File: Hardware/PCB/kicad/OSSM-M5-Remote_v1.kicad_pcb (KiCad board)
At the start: 2 copper layers, 108.5 x 73.1 mm, 13 parts, among them M5-CORE2 M5_CORE2, U1 PCA9685PW, U2 MCP23017_SS, U3 JST-PH-2MM,180

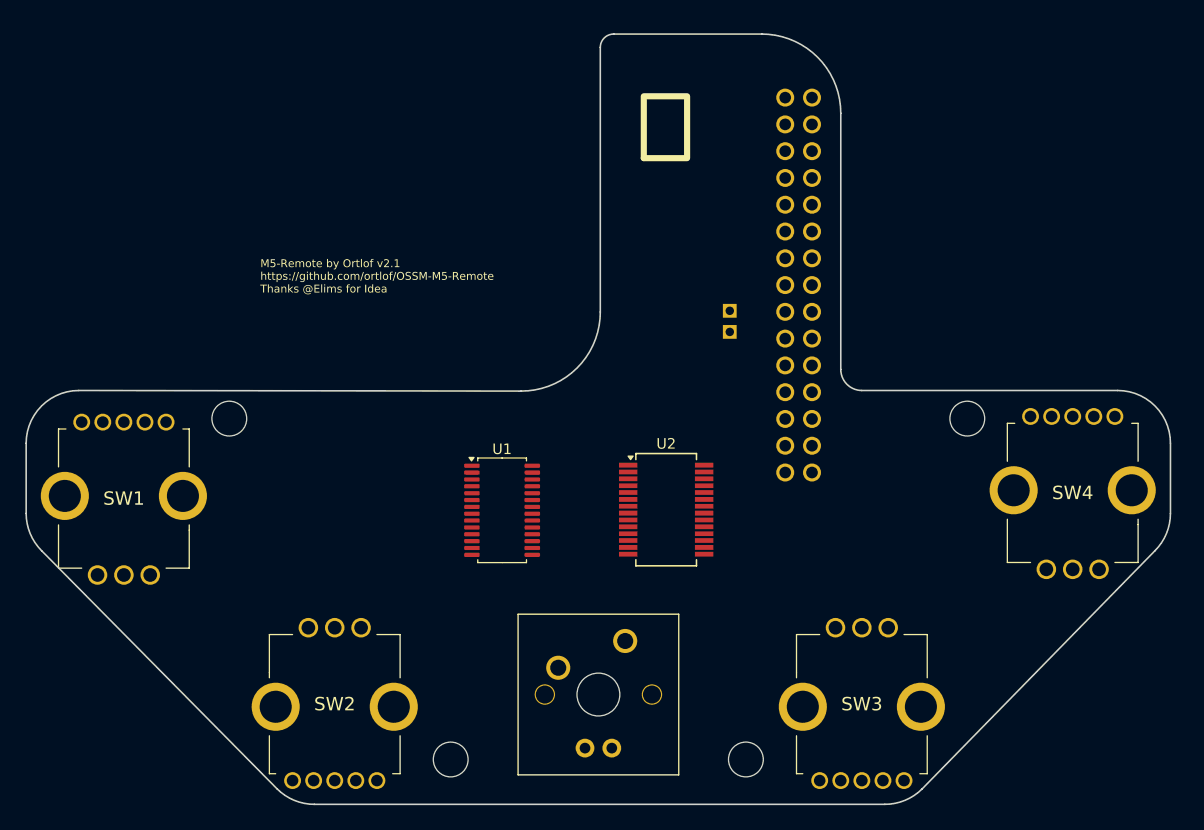
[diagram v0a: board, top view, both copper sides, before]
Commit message: Starting routing
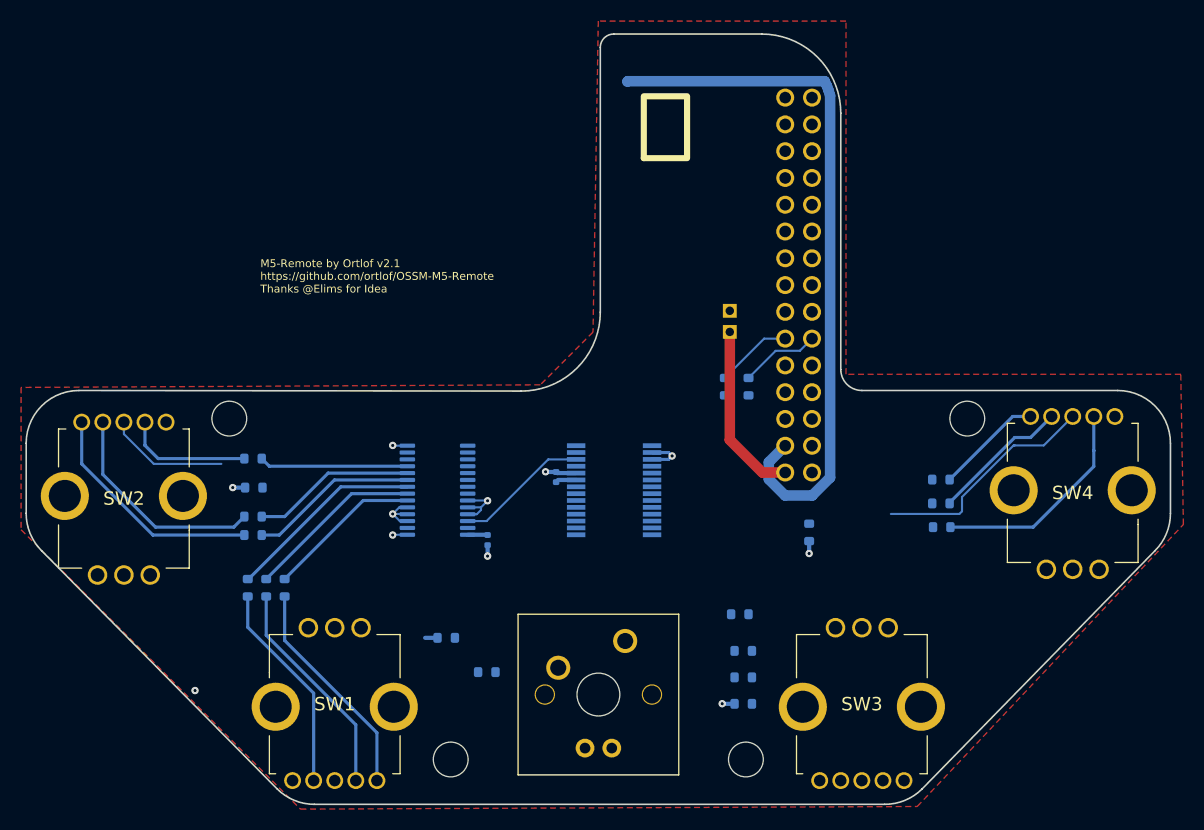
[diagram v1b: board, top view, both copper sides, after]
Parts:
- added C1: 100n, Capacitor_SMD:C_0402_1005Metric, B.Cu at (138.0, 113.7)
- added C2: 100n, Capacitor_SMD:C_0402_1005Metric, B.Cu at (144.5, 107.8)
- added R1: 120R, Resistor_SMD:R_0603_1608Metric, B.Cu at (118.8, 118.2)
- added R10: 120R, Resistor_SMD:R_0603_1608Metric, B.Cu at (162.2, 124.2)
- added R11: 120R, Resistor_SMD:R_0603_1608Metric, B.Cu at (162.2, 126.8)
- added R12: 4k7, Resistor_SMD:R_0603_1608Metric, B.Cu at (162.2, 129.3)
- added R13: 120R, Resistor_SMD:R_0603_1608Metric, B.Cu at (181.0, 108.0)
- added R14: 120R, Resistor_SMD:R_0603_1608Metric, B.Cu at (181.0, 110.2)
- added R15: 120R, Resistor_SMD:R_0603_1608Metric, B.Cu at (181.1, 112.5)
- added R16: 4k7, Resistor_SMD:R_0603_1608Metric, B.Cu at (168.5, 113.0)
- added R17: 120R, Resistor_SMD:R_0603_1608Metric, B.Cu at (137.9, 126.2)
- added R18: 4k7, Resistor_SMD:R_0603_1608Metric, B.Cu at (160.5, 99.2)
- added R19: 4k7, Resistor_SMD:R_0603_1608Metric, B.Cu at (162.8, 99.2)
- added R2: 120R, Resistor_SMD:R_0603_1608Metric, B.Cu at (117.0, 118.2)
- added R3: 120R, Resistor_SMD:R_0603_1608Metric, B.Cu at (115.2, 118.2)
- added R4: 4k7, Resistor_SMD:R_0603_1608Metric, B.Cu at (134.1, 123.0)
- added R5: 120R, Resistor_SMD:R_0603_1608Metric, B.Cu at (115.8, 113.2)
- added R6: 120R, Resistor_SMD:R_0603_1608Metric, B.Cu at (115.8, 111.5)
- added R7: 120R, Resistor_SMD:R_0603_1608Metric, B.Cu at (115.8, 106.0)
- added R8: 4k7, Resistor_SMD:R_0603_1608Metric, B.Cu at (115.8, 108.8)
- added R9: 120R, Resistor_SMD:R_0603_1608Metric, B.Cu at (161.9, 120.8)
- H1: renamed from @HOLE1; value (none) -> MountingHole; footprint (none) -> OSSM-M5-Remote_v1:mounting_hole_3.3mm
- H2: renamed from @HOLE2; value (none) -> MountingHole; footprint (none) -> OSSM-M5-Remote_v1:mounting_hole_3.3mm
- H3: renamed from @HOLE3; value (none) -> MountingHole; footprint (none) -> OSSM-M5-Remote_v1:mounting_hole_3.3mm
- H4: renamed from @HOLE0; value (none) -> MountingHole; footprint (none) -> OSSM-M5-Remote_v1:mounting_hole_3.3mm
- U1, U2: moved to B.Cu
- U4: renamed from U$4; value Val** -> CHERRY-MX-LED
- moved U1 6.42 mm to (133.2, 109.0)
- moved U2 5.27 mm to (150.0, 109.0)
- renumbered SW2 to SW1, SW1 to SW2
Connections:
- net Net-(SW3-SW) renamed /SW3_BUTTON
- net Net-(SW4-SW) renamed /SW4_BUTTON
- net Net-(U2-GPB6) renamed /CHERRY_BUTTON
- M5-CORE2 pad 26: /INTA -> /INTB
- M5-CORE2 pad 5: /INTB -> /INTA
- SW1 pad 1: Net-(SW2--R) -> /LEDD_SW1_R
- SW1 pad 2: Net-(SW2--G) -> /LEDD_SW1_G
- SW1 pad 3: /SW2_BUTTON -> /SW1_BUTTON
- SW1 pad 4: Net-(SW2--B) -> /LEDD_SW1_B
- SW1 pad A: (no net) -> /SW1_ROTA
- SW1 pad B: (no net) -> /SW1_ROTB
- SW1 pad C: (no net) -> GND
- SW1 pad MH1: (no net) -> GND
- SW1 pad MH2: (no net) -> GND
- SW2 pad 1: Net-(SW1--R) -> /LEDD_SW2_R
- SW2 pad 2: Net-(SW1--G) -> /LEDD_SW2_G
- SW2 pad 3: /SW1_BUTTON -> /SW2_BUTTON
- SW2 pad 4: Net-(SW1--B) -> /LEDD_SW2_B
- SW2 pad A: (no net) -> /SW2_ROTB
- SW2 pad B: (no net) -> /SW2_ROTA
- SW2 pad C: (no net) -> GND
- SW2 pad MH1: (no net) -> GND
- SW2 pad MH2: (no net) -> GND
- SW3 pad 1: Net-(SW3--R) -> /LEDD_SW3_R
- SW3 pad 2: Net-(SW3--G) -> /LEDD_SW3_G
- SW3 pad 4: Net-(SW3--B) -> /LEDD_SW3_B
- SW3 pad A: (no net) -> /SW3_ROTB
- SW3 pad B: (no net) -> /SW3_ROTA
- SW3 pad C: (no net) -> GND
- SW3 pad MH1: (no net) -> GND
- SW3 pad MH2: (no net) -> GND
- SW4 pad 1: Net-(SW4--R) -> /LEDD_SW4_R
- SW4 pad 2: Net-(SW4--G) -> /LEDD_SW4_G
- SW4 pad 4: Net-(SW4--B) -> /LEDD_SW4_B
- SW4 pad A: (no net) -> /SW4_ROTA
- SW4 pad B: (no net) -> /SW4_ROTB
- SW4 pad C: (no net) -> GND
- SW4 pad MH1: (no net) -> GND
- SW4 pad MH2: (no net) -> GND
- U1 pad 10: Net-(U1-LED4) -> /LED_SW2_G
- U1 pad 11: Net-(U1-LED5) -> /LED_SW2_B
- U1 pad 12: Net-(U1-LED6) -> /LED_CHERRY
- U1 pad 15: Net-(U1-LED8) -> /LED_SW4_R
- U1 pad 16: Net-(U1-LED9) -> /LED_SW4_G
- U1 pad 17: Net-(U1-LED10) -> /LED_SW4_B
- U1 pad 18: Net-(U1-LED11) -> /LED_SW3_R
- U1 pad 19: Net-(U1-LED12) -> /LED_SW3_G
- U1 pad 20: Net-(U1-LED13) -> /LED_SW3_B
- U1 pad 6: Net-(U1-LED0) -> /LED_SW1_R
- U1 pad 7: Net-(U1-LED1) -> /LED_SW1_G
- U1 pad 8: Net-(U1-LED2) -> /LED_SW1_B
- U1 pad 9: Net-(U1-LED3) -> /LED_SW2_R
- U2 pad 1: Net-(U2-GPB0) -> /SW1_ROTA
- U2 pad 2: Net-(U2-GPB1) -> /SW1_ROTB
- U2 pad 22: Net-(U2-GPA1) -> /SW4_ROTB
- U2 pad 23: Net-(U2-GPA2) -> /SW4_ROTA
- U2 pad 25: Net-(U2-GPA4) -> /SW3_ROTB
- U2 pad 26: Net-(U2-GPA5) -> /SW3_ROTA
- U2 pad 4: Net-(U2-GPB3) -> /SW2_ROTA
- U2 pad 5: Net-(U2-GPB4) -> /SW2_ROTB
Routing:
- net +5V: track 0.00 -> 71.3 mm
- net GND: track 0.00 -> 26.0 mm, vias 0 -> 11
- net /LEDD_SW2_R: track 0.00 -> 22.2 mm
- net /SW4_BUTTON: track 0.00 -> 21.9 mm
- net /LEDD_SW1_R: track 0.00 -> 21.1 mm
- net /LEDD_SW1_G: track 0.00 -> 21.0 mm
- net /LEDD_SW2_G: track 0.00 -> 20.9 mm
- net /LEDD_SW4_B: track 0.00 -> 20.7 mm
- net /LEDD_SW1_B: track 0.00 -> 20.1 mm
- net /SCL: track 0.00 -> 20.0 mm
- net /LED_SW1_B: track 0.00 -> 18.8 mm
- net +BATT: track 0.00 -> 16.8 mm
- net /LED_SW1_G: track 0.00 -> 16.7 mm
- net /LED_SW2_R: track 0.00 -> 16.0 mm
- net /LED_SW2_G: track 0.00 -> 15.5 mm
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- added copper zone on F.Cu, net GND
